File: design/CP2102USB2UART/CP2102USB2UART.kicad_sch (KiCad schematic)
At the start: 13 parts, among them J1 Conn_01x06, J2 UJ2-MIBH-G-SMT-TR, U1 CP2102

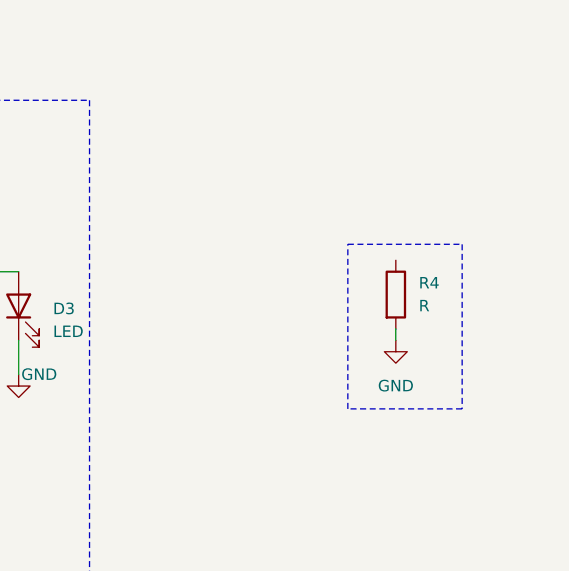
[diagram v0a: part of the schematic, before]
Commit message: bg top and bottom ready
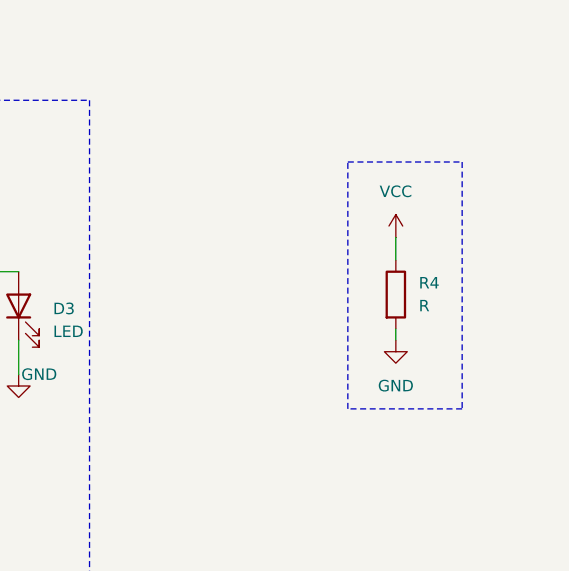
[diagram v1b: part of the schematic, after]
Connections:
- net VCC: now also R4.1
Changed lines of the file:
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@@
+	(wire
+		(pts
+			(xy 229.87 109.22) (xy 229.87 111.76)
+		)
+		(stroke
+			(width 0)
+			(type default)
+		)
+	)
 	(wire
 		(pts
@@
 	)
 	(rectangle
-		(start 224.536 109.982)
+		(start 224.536 100.838)
 		(end 237.236 128.27)
 		(stroke
@@
 					(unit 1)
 				)
+			)
+		)
+	)
+	(symbol
+		(lib_id "power:VCC")
+		(at 229.87 109.22 0)
+		(unit 1)
+		(exclude_from_sim no)
+		(in_bom yes)
+		(on_board yes)
+		(dnp no)
+		(fields_autoplaced yes)
+		(property "Reference" "#PWR014"
+			(at 229.87 113.03 0)
+			(effects
+				(font
+					(size 1.27 1.27)
+				)
+				(hide yes)
+			)
+		)
+		(property "Value" "VCC"
+			(at 229.87 104.14 0)
+			(effects
+				(font
+					(size 1.27 1.27)
+				)
+			)
+		)
+		(property "Footprint" ""
+			(at 229.87 109.22 0)
+			(effects
+				(font
+					(size 1.27 1.27)
+				)
+				(hide yes)
+			)
+		)
+		(property "Datasheet" ""
+			(at 229.87 109.22 0)
+			(effects
+				(font
+					(size 1.27 1.27)
+				)
+				(hide yes)
+			)
+		)
+		(property "Description" "Power symbol creates a global label with name \"VCC\""
+			(at 229.87 109.22 0)
+			(effects
+				(font
+					(size 1.27 1.27)
+				)
+				(hide yes)
+			)
+		)
+		(pin "1"
+		)
+		(instances
+			(project "CP2102USB2UART"
+				(path "/4c3b105e-46d9-4f53-a989-3f2215a086af"
+					(reference "#PWR014")
+					(unit 1)
+				)

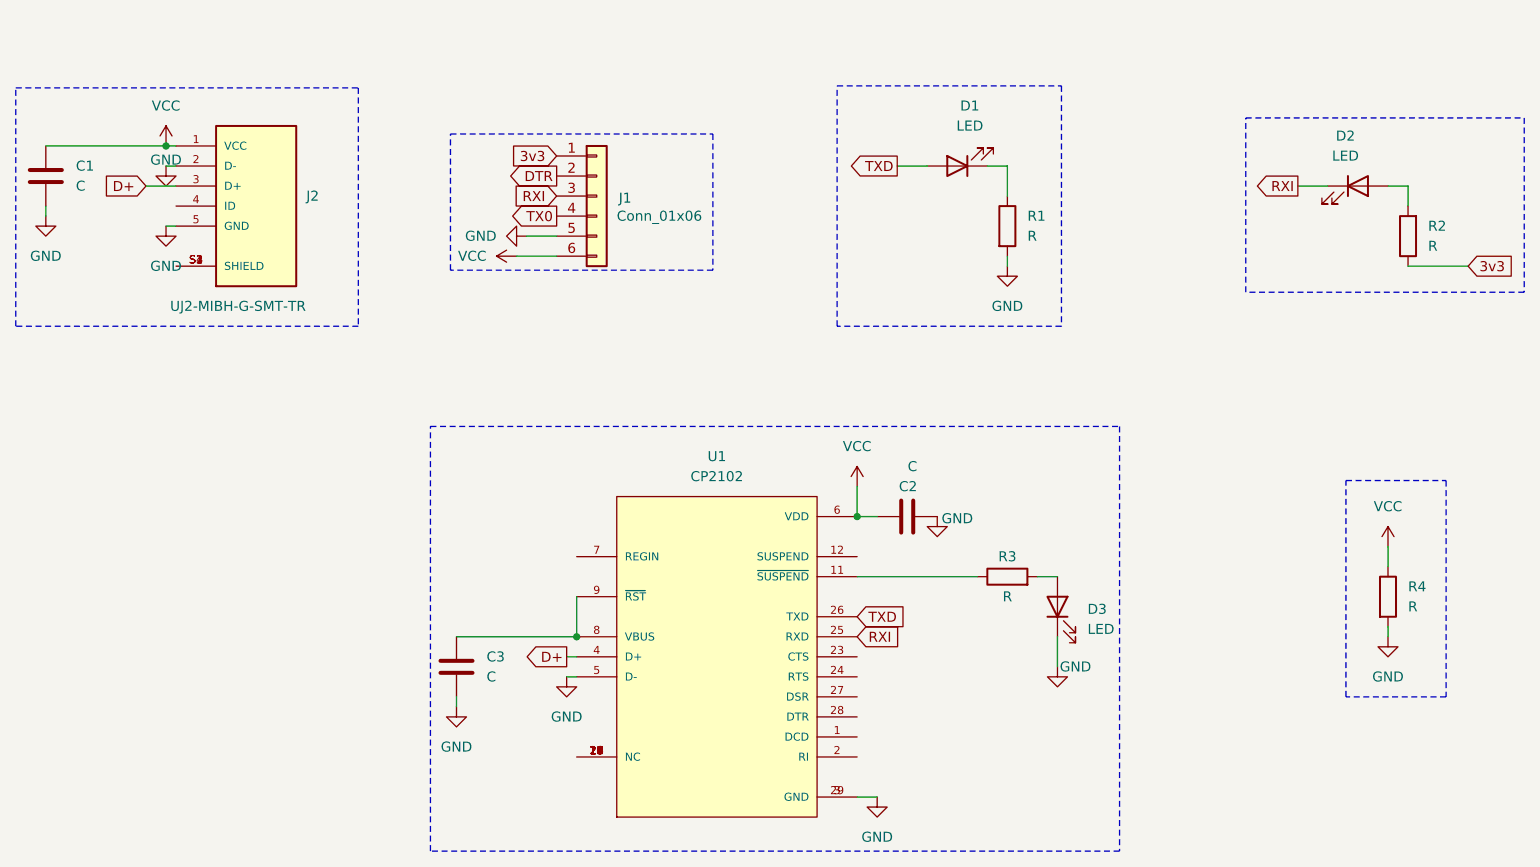
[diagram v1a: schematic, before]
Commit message: end of retroengineering
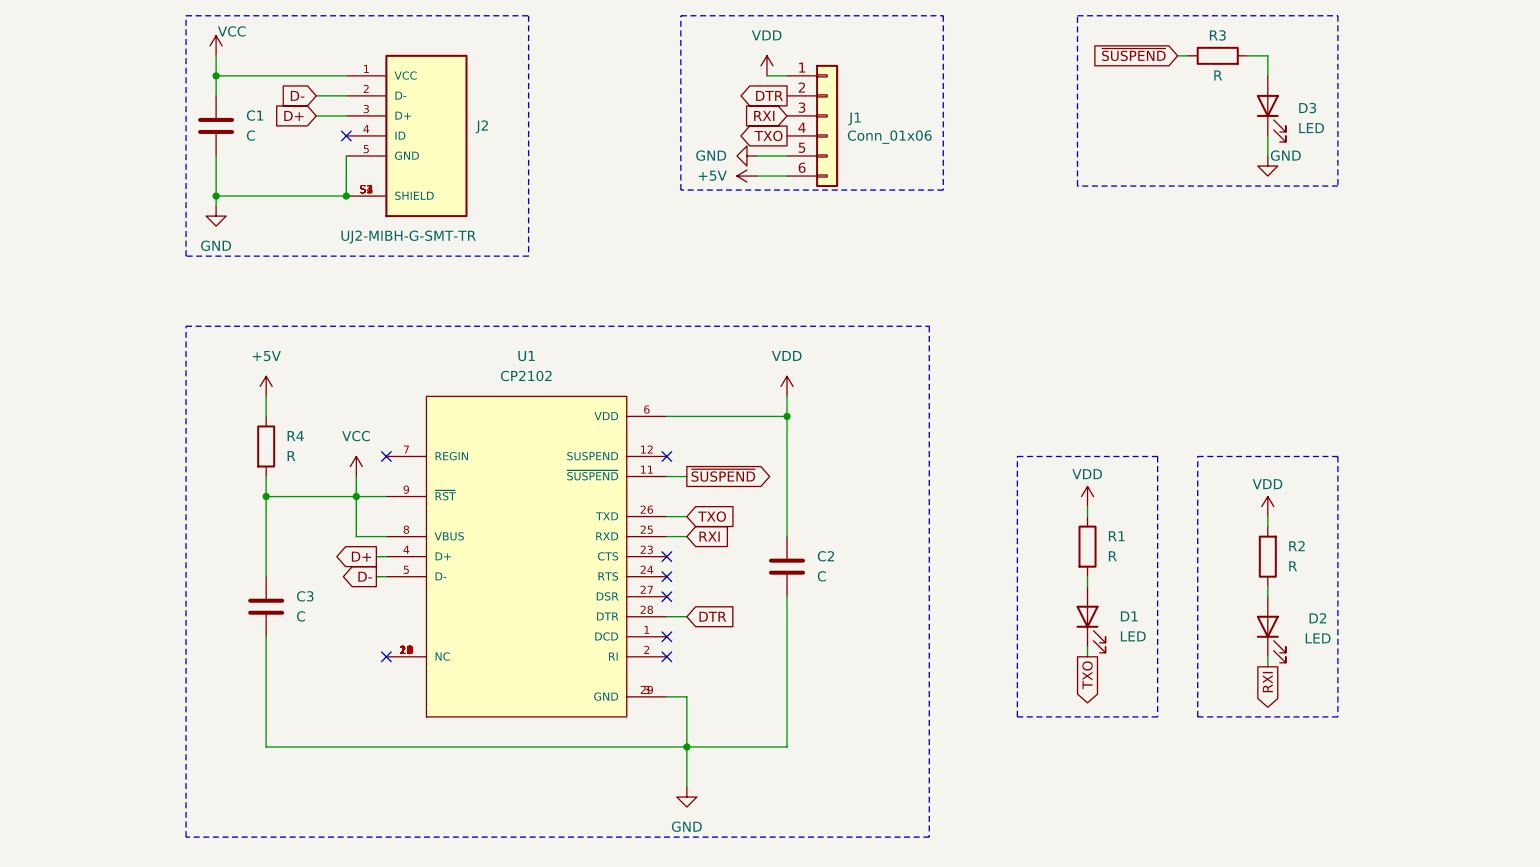
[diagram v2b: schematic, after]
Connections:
- net TX0 is gone; now on net TXO: J1.4 (Pin_4)
- net DTR: now also U1.28 (DTR)
- net GND: now also J2.S1 (SHIELD), J2.S2 (SHIELD), J2.S3 (SHIELD), J2.S4 (SHIELD); no longer J2.2 (D-), R1.2, R4.2, U1.5 (D-)
- net VCC: now also C3.1, R4.2, U1.8 (VBUS), U1.9 (~{RST}); no longer C2.1, J1.6 (Pin_6), R4.1, U1.6 (VDD)
- net ~{SUSPEND}: now reaches R3.1, U1.11 (~{SUSPEND})
- net TXO: now reaches D1.1 (K)
- net TXO: now also U1.26 (TXD); no longer R1.1
- net at D2.2 (A): now also R2.1; no longer R2.2
- net 3v3 renamed VDD
- net VDD: now also C2.1, R1.1, R2.2, U1.6 (VDD); no longer R2.1
- net TXD: no longer names the net of D1.2 (A)
- net TXD: now also R1.2; no longer U1.26 (TXD)
- new net +5V: J1.6 (Pin_6), R4.1
- new net D-: J2.2 (D-), U1.5 (D-)
- no-connect marks 0 -> 9
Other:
- moved on the sheet: C1, C2, C3, D1, D2, D3, J1, J2, R1, R2, R3, R4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
